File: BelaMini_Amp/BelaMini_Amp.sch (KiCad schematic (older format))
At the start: 17 parts, among them J3 Conn_01x03_Female, J4 Conn_01x03_Female, SW1 SW_Push, SW2 SW_Push, SW3 SW_Push, U1 BelaMini

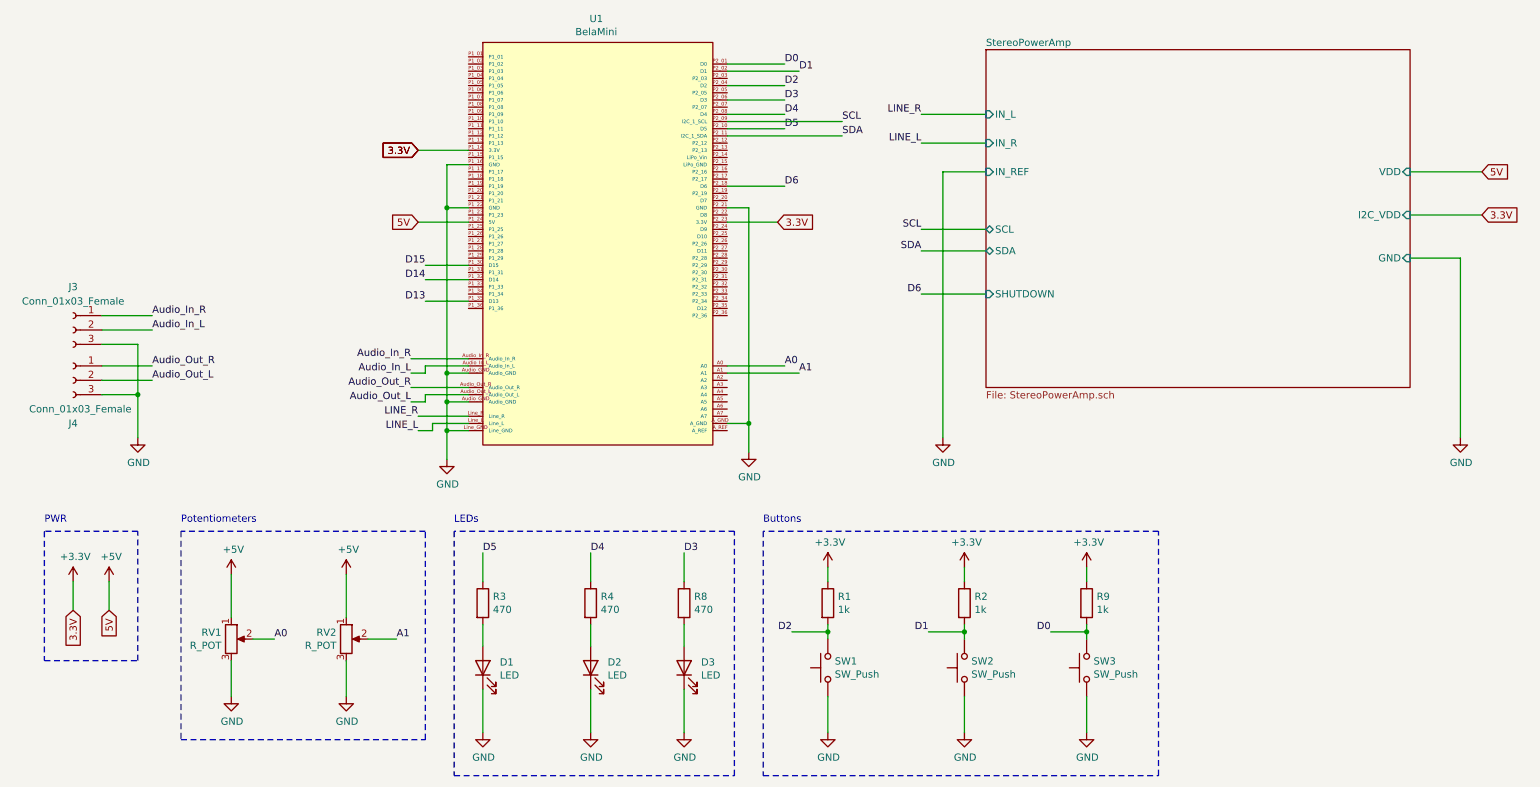
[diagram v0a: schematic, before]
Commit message: Updated example
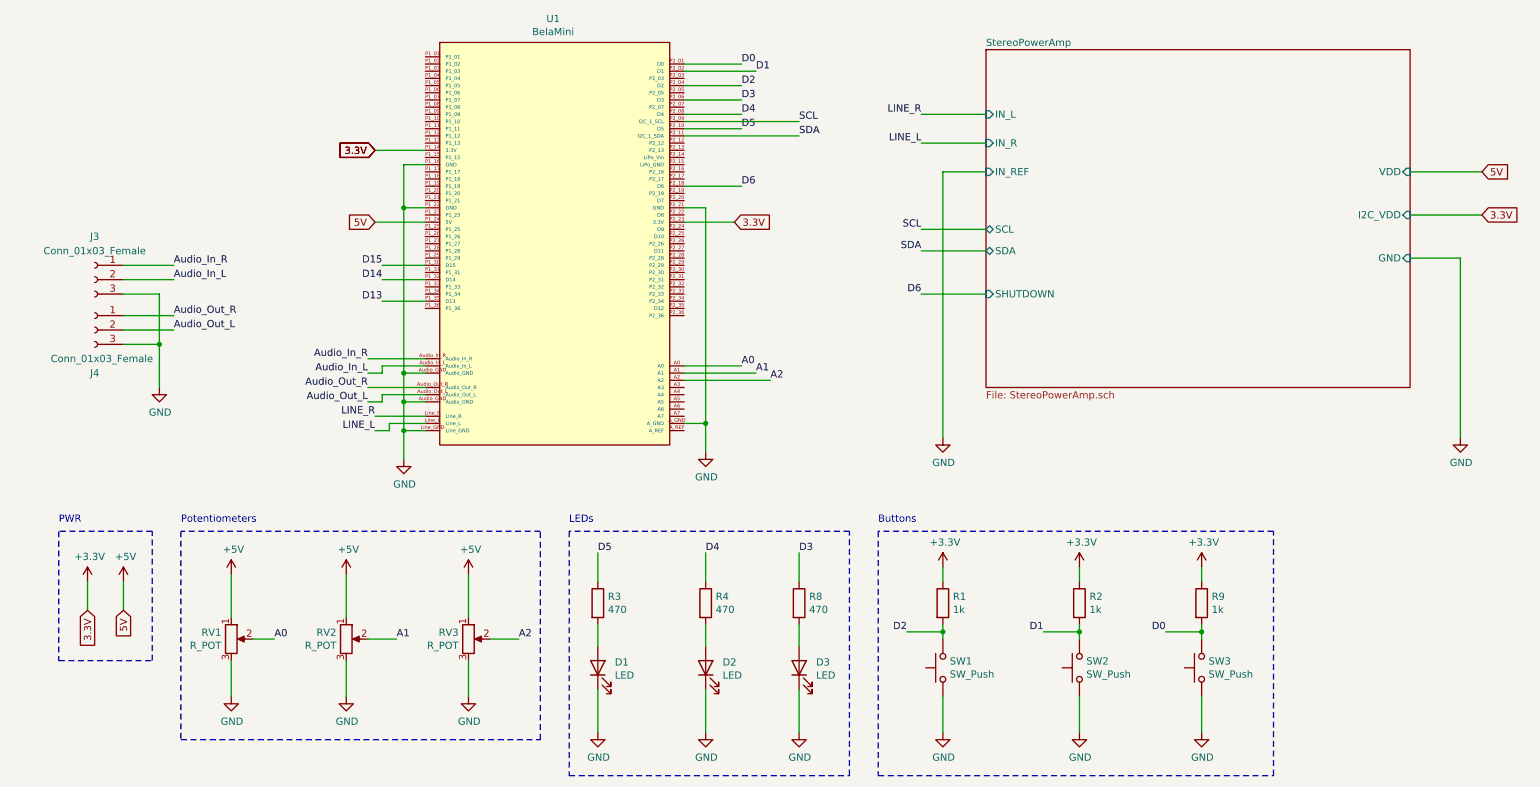
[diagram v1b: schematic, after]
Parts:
- added RV3: R_POT, Potentiometer_THT:Potentiometer_Alpha_RD901F-40-00D_Single_Vertical, symbol Device:R_POT
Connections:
- net +5V: now also RV3.1
- net GND: now also RV3.3
- net A2: now reaches U1.A2
- net A2: now also RV3.2
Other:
- moved on the sheet: D1, D2, D3, J3, J4, R1, R2, R3, R4, R8, R9, SW1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
